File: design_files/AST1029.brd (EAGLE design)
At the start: 10 x 10 mm, 4 parts, among them J1 SM05B, SW1 PCM12SMTR

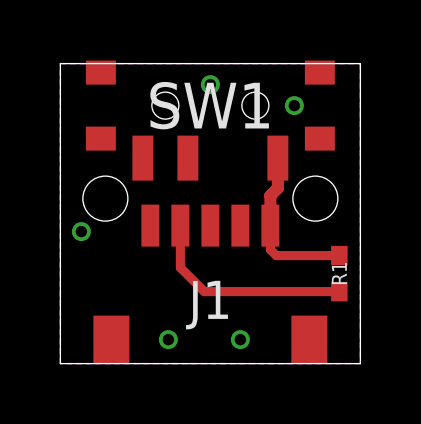
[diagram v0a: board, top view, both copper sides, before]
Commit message: updates:
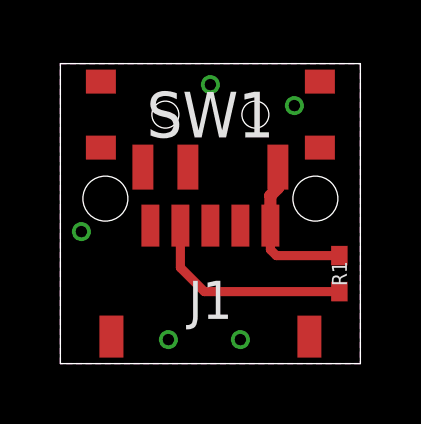
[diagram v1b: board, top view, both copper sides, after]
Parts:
- J1: device tinycircuits:JST_SH_5X1 -> tinycircuits:JST_SH_5X1_EDGE
- moved SW1 0.30 mm to (20.0, 18.3)
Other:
- board text added: "AST1029 R1"
- board text added: "Switch"
- board text added: "Wireling Small Switch"
- board text removed: "AST1029"
- board text removed: "Switch Board"
- board text removed: "Switch R1"
